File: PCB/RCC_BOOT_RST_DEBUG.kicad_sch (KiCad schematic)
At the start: 21 parts, among them U2 STM32MP157FABx, Y1 ECS-2520MVQ-240

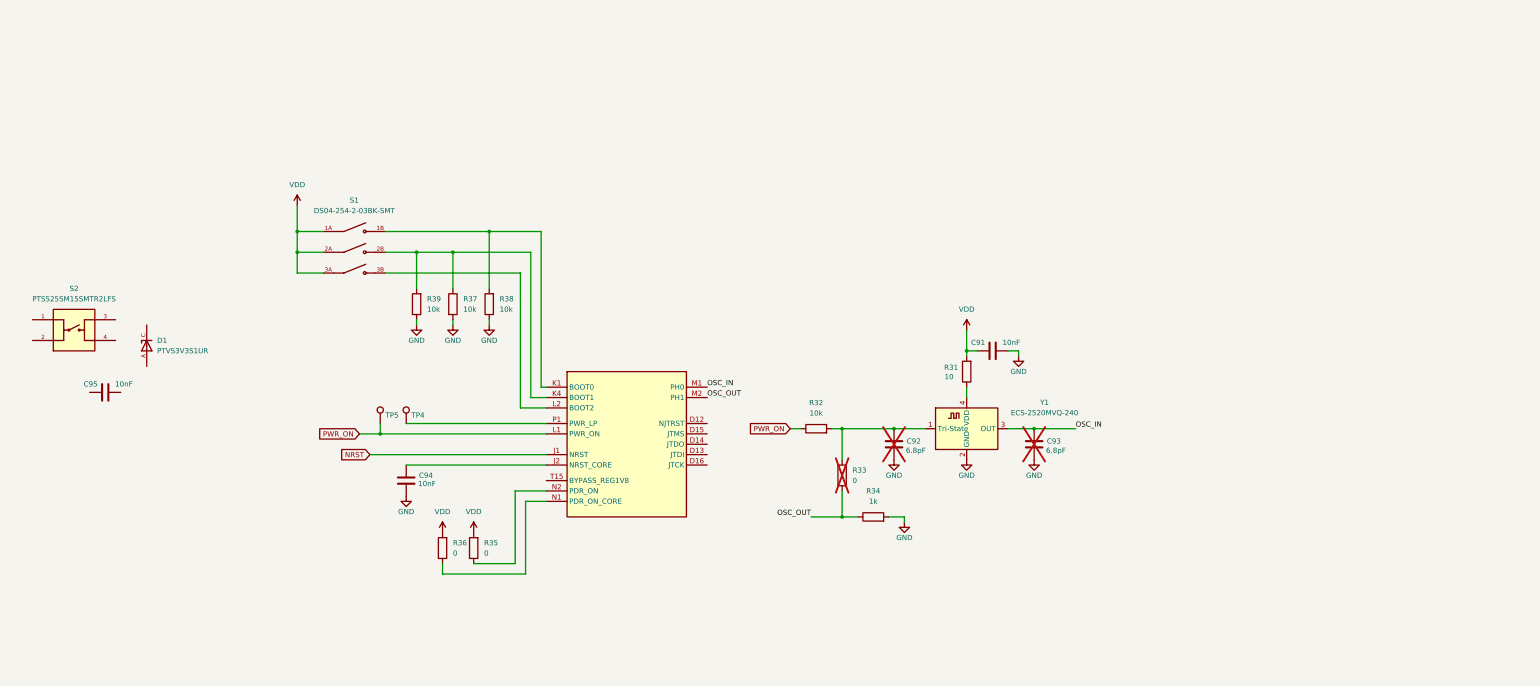
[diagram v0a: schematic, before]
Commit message: Look like MPU done
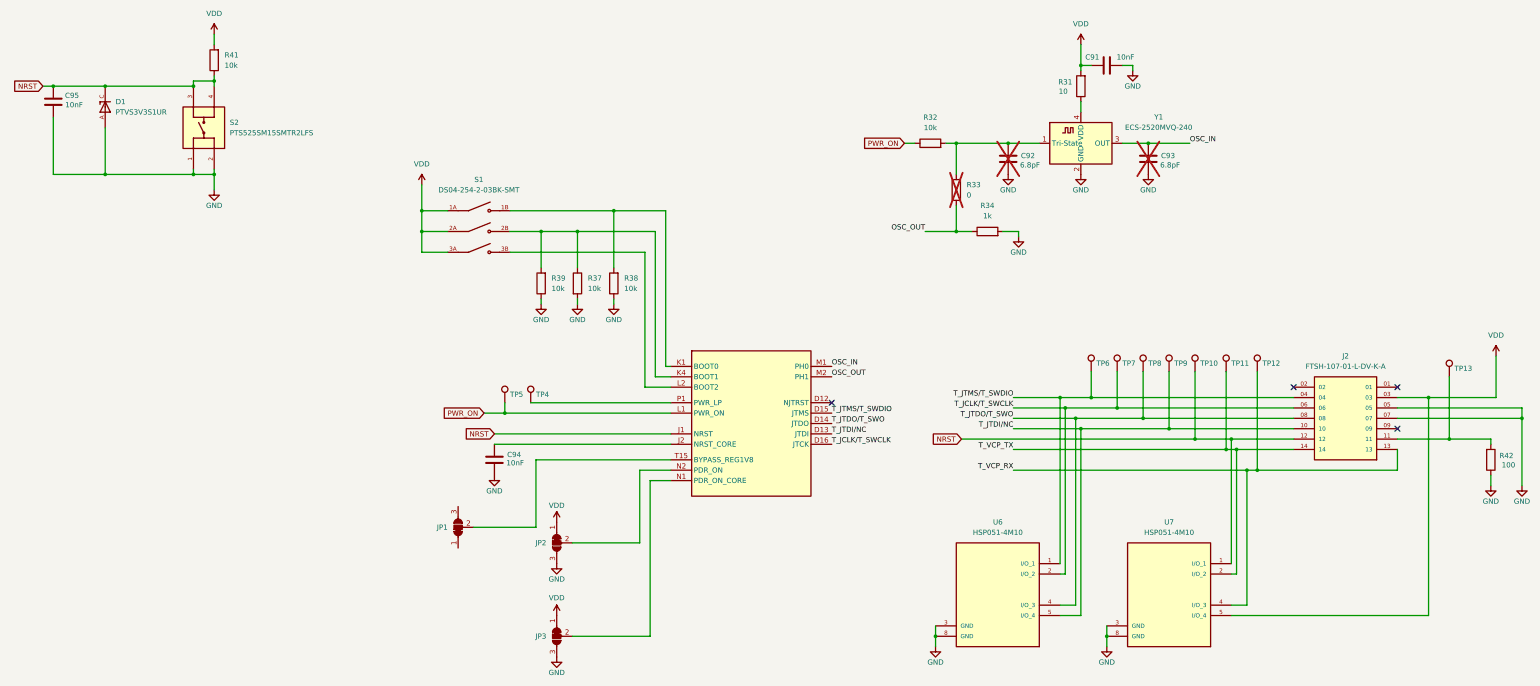
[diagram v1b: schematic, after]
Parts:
- removed R35, R36: 0, symbol Device:R
- added J2: FTSH-107-01-L-DV-K-A, FTSH-107-01-L-DV-K-A:SAMTEC_FTSH-107-01-L-DV-K-A, symbol FTSH-107-01-L-DV-K-A:FTSH-107-01-L-DV-K-A
- added JP1, JP2, JP3: SolderJumper_3_Bridged12, Jumper:SolderJumper-3_P1.3mm_Bridged12_Pad1.0x1.5mm, symbol Jumper:SolderJumper_3_Bridged12
- added R41: 10k, symbol Device:R
- added R42: 100, symbol Device:R
- added TP10, TP11, TP12, TP13, TP6, TP7, TP8, TP9: TestPoint, TestPoint:TestPoint_Pad_D1.0mm, symbol Connector:TestPoint
- added U6, U7: HSP051-4M10, HSP051-4M10:IC_HSP051-4M10, symbol HSP051-4M10:HSP051-4M10
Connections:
- net GND: now also C95.1, D1.A, S2.1, S2.2, J2.05, J2.07, JP2.3 (B), JP3.3 (B), R42.1, U6.3 (GND), U6.8 (GND), U7.3 (GND), U7.8 (GND)
- net NRST: now also C95.2, D1.C, S2.3, S2.4, J2.12, R41.1, TP10.1, U7.1 (I/O_1), U7.10 (NC)
- net VDD: now also J2.03, JP2.1 (A), JP3.1 (A), R41.2, U7.5 (I/O_4), U7.6 (NC)
- net T_JTDI/NC: now reaches U2.D13 (JTDI)
- net T_JTDI/NC: now also J2.10, TP9.1, U6.5 (I/O_4), U6.6 (NC)
- net T_JTDO/T_SWO: now reaches U2.D14 (JTDO)
- net T_JTDO/T_SWO: now also J2.08, TP8.1, U6.4 (I/O_3), U6.7 (NC)
- net T_JTMS/T_SWDIO: now reaches U2.D15 (JTMS)
- net T_JTMS/T_SWDIO: now also J2.04, TP6.1, U6.1 (I/O_1), U6.10 (NC)
- net T_JCLK/T_SWCLK: now reaches U2.D16 (JTCK)
- net T_JCLK/T_SWCLK: now also J2.06, TP7.1, U6.2 (I/O_2), U6.9 (NC)
- net at U2.N1 (PDR_ON_CORE): now also JP3.2 (C)
- net at U2.N2 (PDR_ON): now also JP2.2 (C)
- net at U2.T15 (BYPASS_REG1V8): now also JP1.2 (C)
- new net: J2.11, R42.2, TP13.1
- new net T_VCP_RX: J2.13, TP12.1, U7.4 (I/O_3), U7.7 (NC)
- new net T_VCP_TX: J2.14, TP11.1, U7.2 (I/O_2), U7.9 (NC)
- no-connect marks 0 -> 4
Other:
- moved on the sheet: C91, C92, C93, C94, C95, D1, R31, R32, R33, R34, R37, R38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
